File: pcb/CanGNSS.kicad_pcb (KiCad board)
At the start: 2 copper layers, 66.4 x 36.8 mm, 18 parts, among them IC101 ATTINY3224-SS, P101 Debug, P103 CAN, U101 MCP2515, U102 TJA1050, U103 NCP1117ST50T3G, U104 neo-m8n-module, X101 8MHz

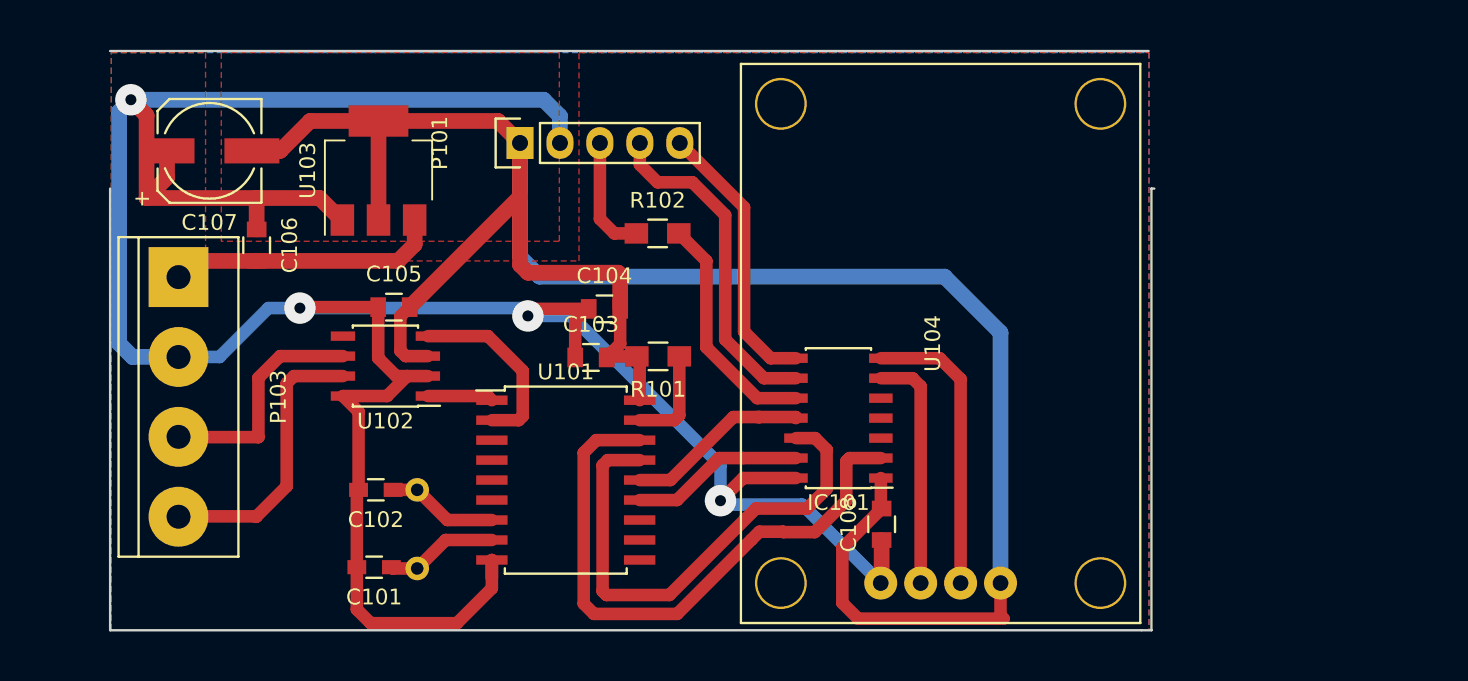
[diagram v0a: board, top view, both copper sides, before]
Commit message: Updated board and config
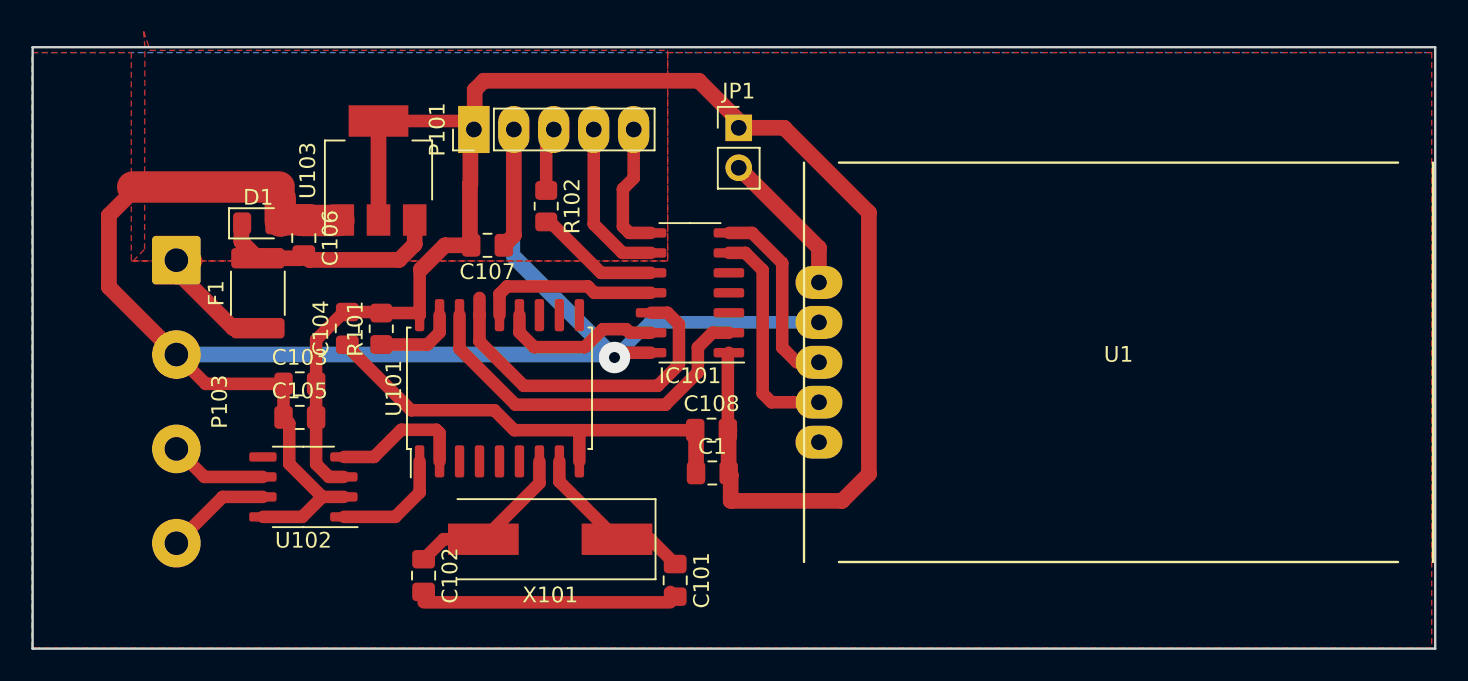
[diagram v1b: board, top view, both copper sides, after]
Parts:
- removed U104: neo-m8n-module, Divers:neo-m8n-module
- added C1: 10uF, Capacitor_SMD:C_0805_2012Metric_Pad1.18x1.45mm_HandSolder, F.Cu at (144.3, 126.9)
- added D1: D, Diode_SMD:D_0805_2012Metric_Pad1.15x1.40mm_HandSolder, F.Cu at (115.4, 111.0)
- added F1: Polyfuse_Small, Fuse:Fuse_1812_4532Metric_Pad1.30x3.40mm_HandSolder, F.Cu at (115.4, 115.5)
- added JP1: Jumper_2_Bridged, Connector_PinHeader_2.54mm:PinHeader_1x02_P2.54mm_Vertical, F.Cu at (145.9, 104.9)
- added U1: neo-m8n-module-mini, iebSpecials:neo-m8n-module-mini, F.Cu at (170.1, 119.9)
- C101, C102: footprint Resistors_SMD:R_0603_HandSoldering -> Capacitor_SMD:C_0805_2012Metric_Pad1.18x1.45mm_HandSolder
- C103, C104, C105, C106, C108: footprint Capacitors_SMD:C_0805 -> Capacitor_SMD:C_0805_2012Metric_Pad1.18x1.45mm_HandSolder
- C107: value 100uF -> 10uF; footprint Capacitors_SMD:c_elec_6.3x5.7 -> Capacitor_SMD:C_0805_2012Metric_Pad1.18x1.45mm_HandSolder
- IC101: footprint Housings_SOIC:SOIC-14_3.9x8.7mm_Pitch1.27mm -> Package_SO:SO-14_3.9x8.65mm_P1.27mm
- P101: footprint Pin_Headers:Pin_Header_Straight_1x05 -> Connector_PinHeader_2.54mm:PinHeader_1x05_P2.54mm_Vertical
- P103: footprint Connect:bornier4 -> Connector_Wire:SolderWire-1.5sqmm_1x04_P6mm_D1.7mm_OD3mm
- R101: footprint Resistors_SMD:R_0805_HandSoldering -> Resistor_SMD:R_0805_2012Metric_Pad1.20x1.40mm_HandSolder
- R102: value 10K -> 470R; footprint Resistors_SMD:R_0805_HandSoldering -> Resistor_SMD:R_0805_2012Metric_Pad1.20x1.40mm_HandSolder
- U101: footprint Housings_SOIC:SOIC-18W_7.5x11.6mm_Pitch1.27mm -> Package_SO:SOIC-18W_7.5x11.6mm_P1.27mm
- U102: footprint Housings_SOIC:SOIC-8_3.9x4.9mm_Pitch1.27mm -> Package_SO:SO-8_3.9x4.9mm_P1.27mm
- U103: footprint TO_SOT_Packages_SMD:SOT-223-3Lead_TabPin2 -> Package_TO_SOT_SMD:SOT-223-3_TabPin2
- X101: value 8MHz -> 16MHz; footprint Crystals:Resonator-2pin_w10.0mm_h5.0mm -> Crystal:Crystal_SMD_HC49-SD; moved to F.Cu
- moved C101 19.2 mm to (141.9, 133.7), turned to -90 degrees
- moved C107 18.7 mm to (130.0, 112.4), turned to 180 degrees
- moved C103 18.6 mm to (118.0, 121.2)
- moved R101 17.7 mm to (123.2, 117.7), turned to 90 degrees
- moved C104 16.4 mm to (121.1, 117.7), turned to 90 degrees
- moved C108 12.4 mm to (144.2, 124.2), turned to 0 degrees
- moved IC101 12.4 mm to (142.8, 115.4)
- moved U102 9.29 mm to (118.3, 127.8)
- moved C105 9.22 mm to (118.0, 123.4)
- moved P103 8.70 mm to (110.2, 113.4)
- moved X101 8.66 mm to (134.0, 131.1), turned to 180 degrees
- moved R102 7.29 mm to (133.7, 109.9), turned to -90 degrees
- moved U101 7.20 mm to (130.7, 121.5), turned to 90 degrees
- moved C102 6.24 mm to (125.9, 133.4), turned to -90 degrees
- moved P101 3.06 mm to (129.1, 105.1)
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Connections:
- C106 pad 2: 12v -> Net-(D1-K)
- IC101 pad 3: (no net) -> unconnected-(IC101-PA5(AIN5/OUT)-Pad3)
- IC101 pad 4: (no net) -> unconnected-(IC101-PA6(AIN6)-Pad4)
- IC101 pad 5: (no net) -> unconnected-(IC101-PA7(AIN7/EVOUTA)-Pad5)
- U101 pad 10: (no net) -> unconnected-(U101-RX1BF-Pad10)
- U101 pad 11: (no net) -> unconnected-(U101-RX0BF-Pad11)
- U101 pad 12: (no net) -> unconnected-(U101-INT-Pad12)
- U101 pad 3: (no net) -> unconnected-(U101-CLKOUT-Pad3)
- U101 pad 4: (no net) -> unconnected-(U101-TX0RTS-Pad4)
- U101 pad 5: (no net) -> unconnected-(U101-TX1RTS-Pad5)
- U101 pad 6: (no net) -> unconnected-(U101-TX2RTS-Pad6)
- U102 pad 5: (no net) -> unconnected-(U102-Vref-Pad5)
- U103 pad 3: 12v -> Net-(D1-K)
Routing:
- net 5V: track 142.1 -> 112.6 mm
- net GND: track 188.7 -> 164.2 mm, vias 4 -> 1
- net Net-(D1-K): track 0.00 -> 14.8 mm
- net CANCS: track 38.3 -> 23.6 mm
- net CANH: track 18.0 -> 6.72 mm
- net DEBUG_RX: track 21.6 -> 10.4 mm
- net MISO: track 32.4 -> 21.8 mm
- net 5Vswitched: track 0.00 -> 9.41 mm
- net DEBUG_TX: track 17.7 -> 8.42 mm
- net 12v: track 17.4 -> 8.84 mm
- net CANL: track 14.8 -> 6.24 mm
- net Net-(IC101-(UDPI/RESET)_PA0): track 15.0 -> 8.01 mm
- net GPSTX: track 18.6 -> 12.3 mm
- net Net-(U101-OSC2): track 7.08 -> 10.8 mm
- net Net-(U101-OSC1): track 7.17 -> 10.8 mm
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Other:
- board size 66.4 x 36.8 mm -> 89.2 x 38.3 mm
- net class Default removed
